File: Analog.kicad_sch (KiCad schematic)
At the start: 33 parts, among them J5 Conn_01x06, U6 MCP4725xxx-xCH, U7 MCP602, U8 MCP602

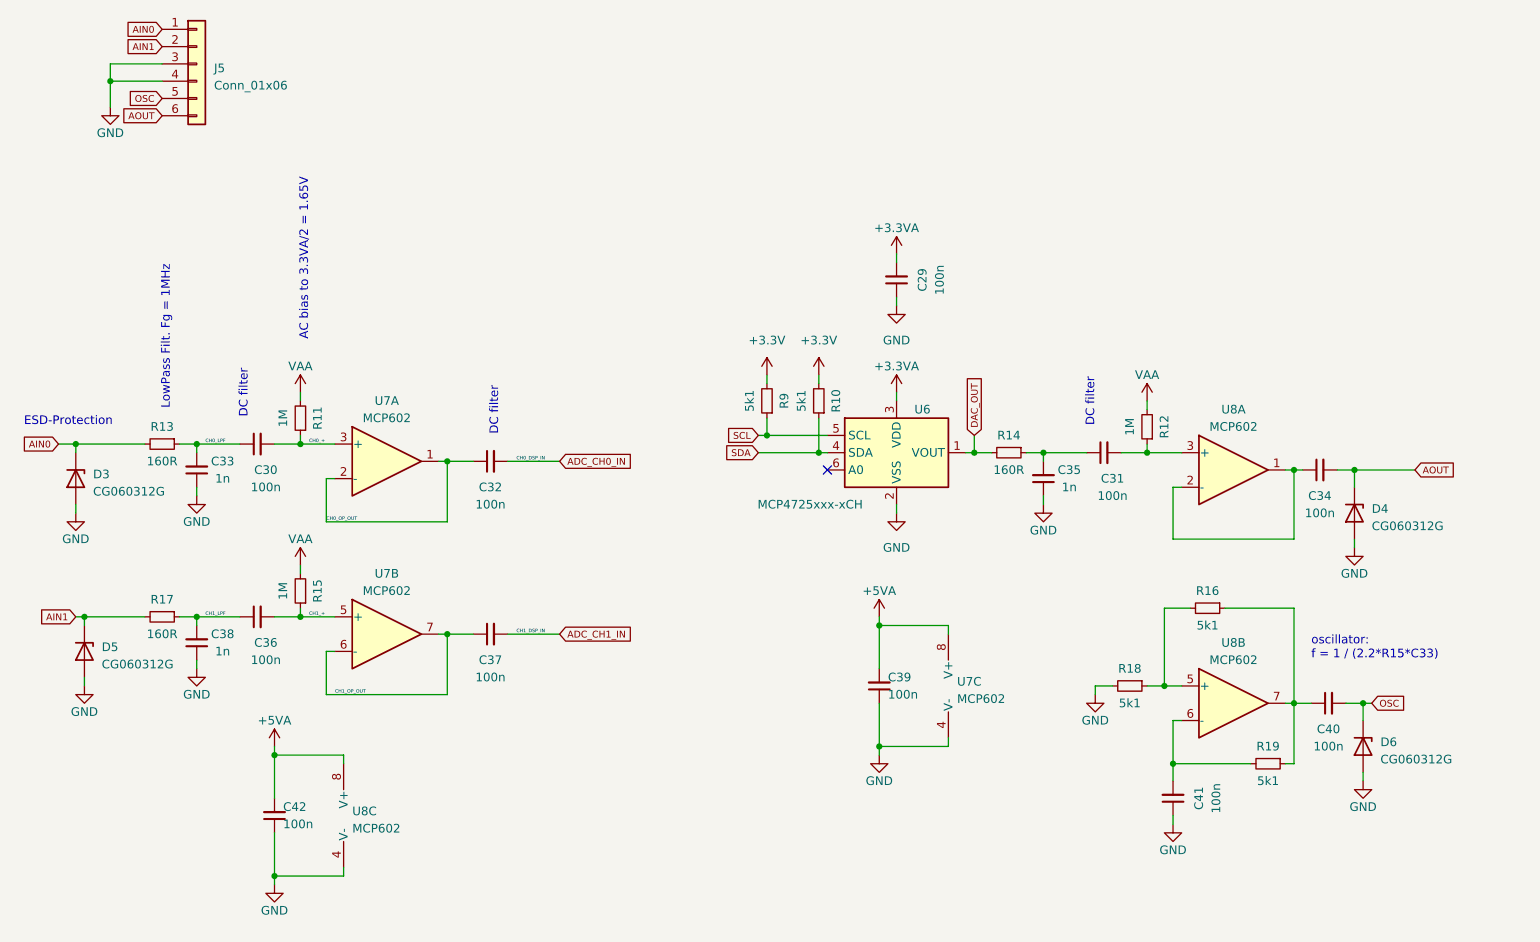
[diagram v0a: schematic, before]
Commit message: cleanup
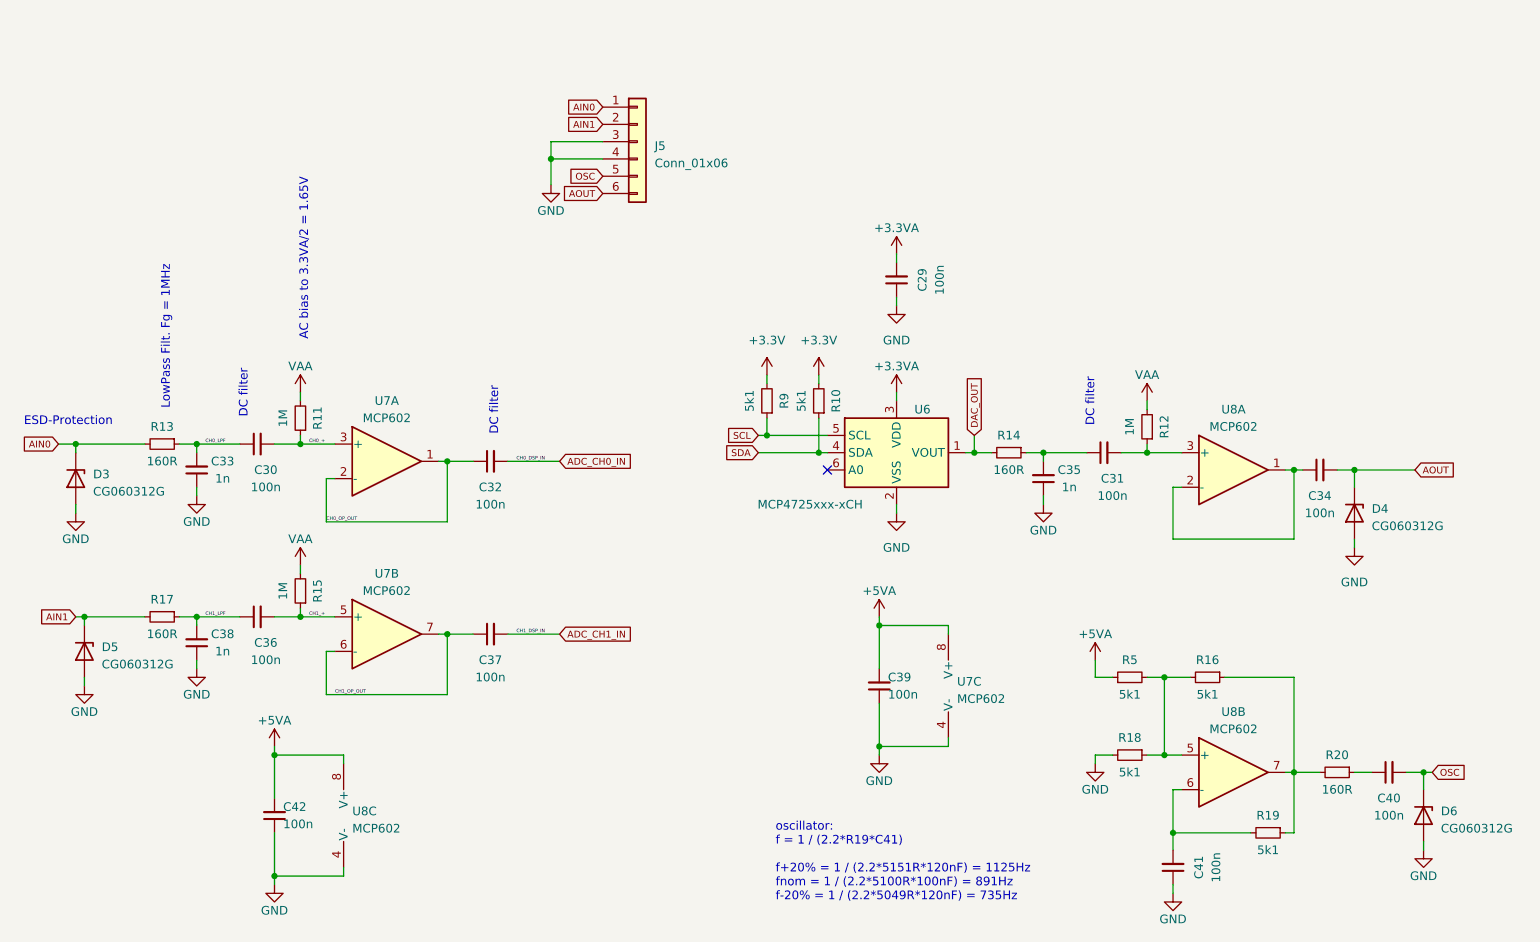
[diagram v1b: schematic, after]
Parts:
- added R20: 160R, Resistor_SMD:R_0603_1608Metric_Pad0.98x0.95mm_HandSolder, symbol Device:R_Small
- added R5: 5k1, Resistor_SMD:R_0603_1608Metric_Pad0.98x0.95mm_HandSolder, symbol Device:R_Small
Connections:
- net +5VA: now also R5.1
- net at R16.2, R18.1, U8.5 (+): now also R5.2
- net at R16.1, R19.1, U8.7: now also R20.2; no longer C40.1
- new net: C40.1, R20.1
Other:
- note added: "oscillator: f = 1 / (2.2*R19*C41) f+20% = 1 / (2.2*5151R*120nF) = 1125Hz fnom = 1 / (2.2*5100R*100nF) = 891Hz f-20% = 1 / (2.2*5049R*120nF) = 735Hz"
- note removed: "oscillator: f = 1 / (2.2*R15*C33)"
- moved on the sheet: C40, C41, D6, J5, R16, R18, R19, U8B
